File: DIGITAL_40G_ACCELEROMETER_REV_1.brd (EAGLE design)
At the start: 19 x 38 mm, 18 parts, among them IC1 ADIS16500AMLZ, IC2 LTC6820IUD#PBF, IC3 LDL1117S33R, T1 782482_33VC

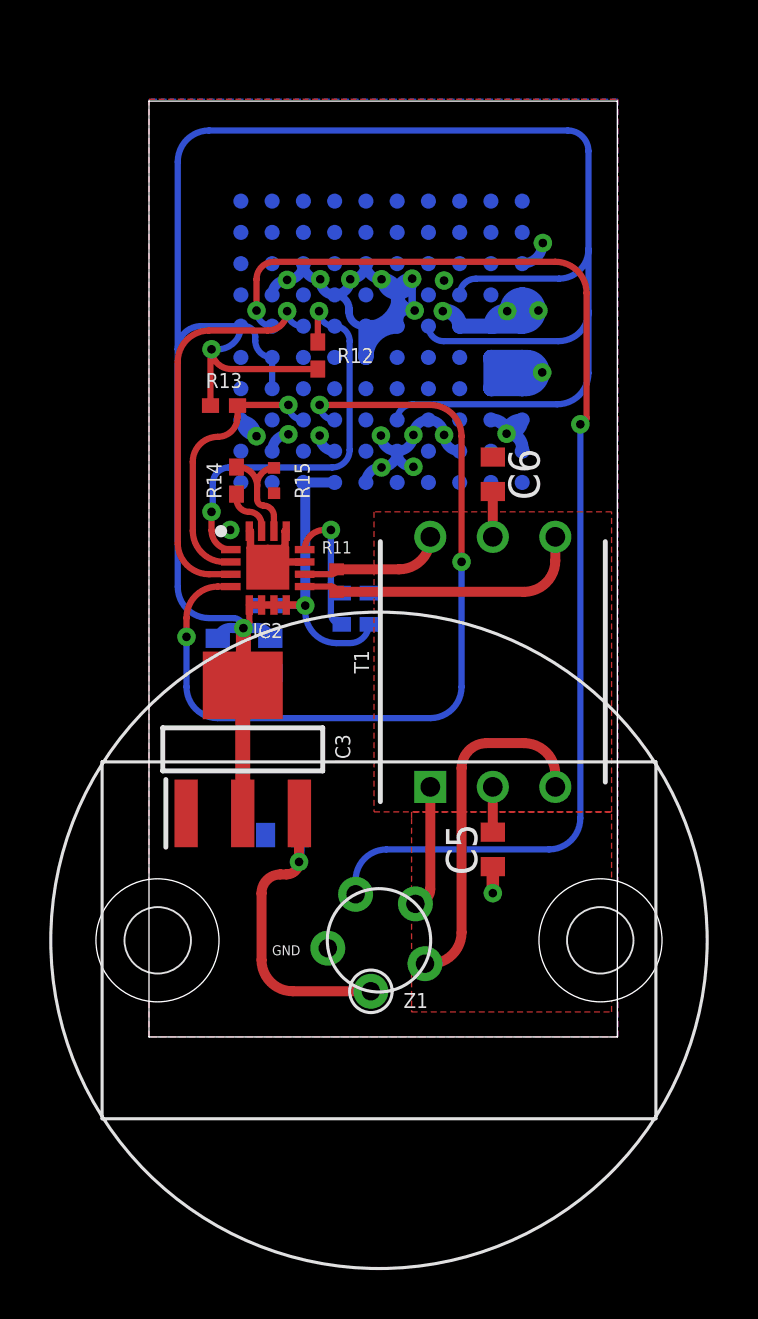
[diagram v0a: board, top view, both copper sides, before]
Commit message: Second Draft of Digital 40G Layout. Ready for review.
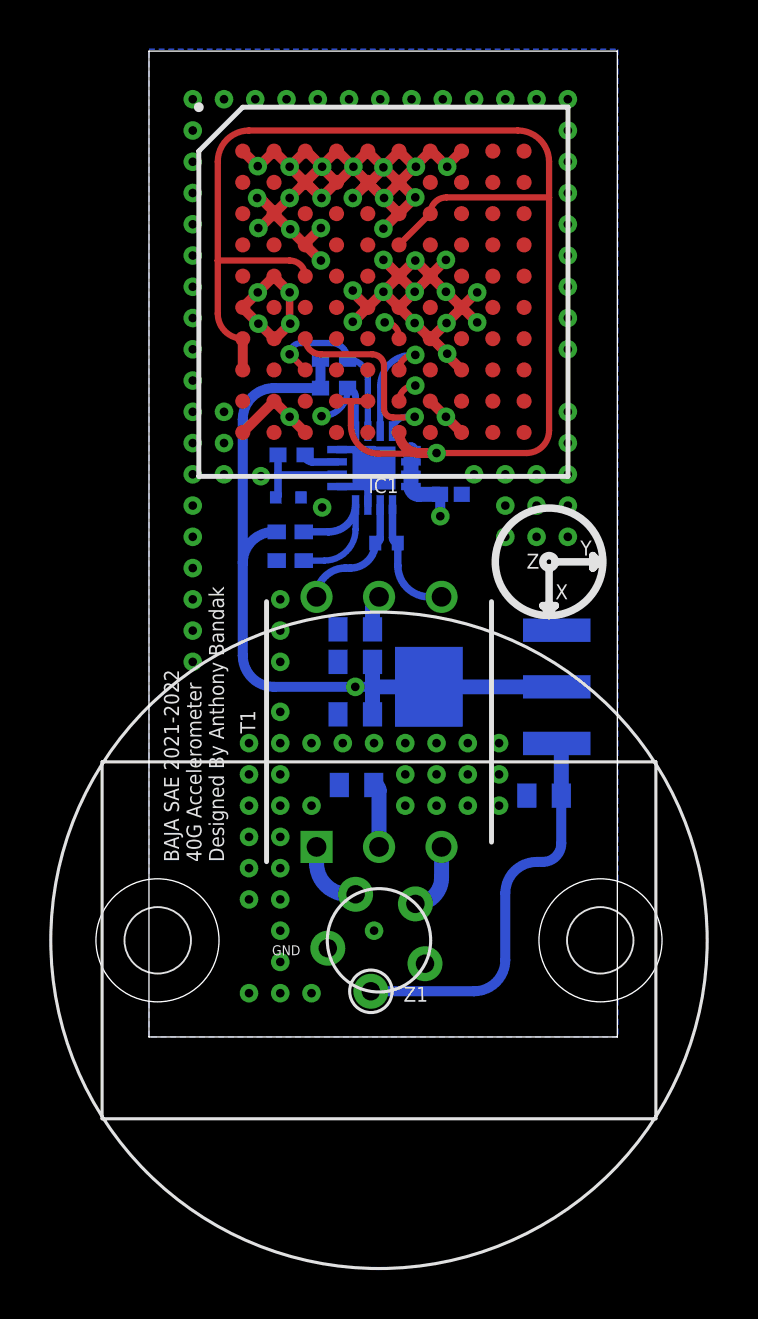
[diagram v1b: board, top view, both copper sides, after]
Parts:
- moved C1 10.7 mm to (16.1, 9.80)
- moved IC3 10.5 mm to (14.0, 14.2), flipped to the bottom, turned to 0 degrees
- moved C4 8.71 mm to (12.3, 22.0), turned to 180 degrees
- moved C6 8.42 mm to (8.38, 16.6), flipped to the bottom, turned to 0 degrees
- moved C5 6.12 mm to (8.43, 10.2), flipped to the bottom, turned to 0 degrees
- moved IC2 5.93 mm to (9.14, 23.1), flipped to the bottom, turned to 270 degrees
- moved C2 5.59 mm to (8.38, 15.2), turned to 0 degrees
- moved T1 5.23 mm to (9.35, 12.8)
- moved R13 4.85 mm to (7.52, 27.5), flipped to the bottom, turned to 0 degrees
- moved R17 4.59 mm to (5.74, 20.5), turned to 0 degrees
- moved C3 4.20 mm to (8.38, 13.1), turned to 0 degrees
- moved R16 2.95 mm to (5.74, 19.4), turned to 0 degrees
- moved R11 2.54 mm to (9.65, 20.1), flipped to the bottom, turned to 0 degrees
- moved R14 2.47 mm to (5.79, 23.6), flipped to the bottom, turned to 0 degrees
- moved IC1 2.03 mm to (9.53, 30.3), flipped to the top, turned to 0 degrees
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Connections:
- net DR: now also Z1.3; no longer Z1.5
- net IM: now also Z1.4; no longer Z1.3
- net IP: now also Z1.5; no longer Z1.4
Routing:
- net CS: track 34.7 -> 7.94 mm, vias 3 -> 1
- net DR: track 48.6 -> 35.0 mm, vias 2 -> 1
- net SCK: track 16.3 -> 4.69 mm
- net IM: track 14.0 -> 2.76 mm
- net IMBOARD: track 11.8 -> 4.86 mm
- net MOSI: track 16.6 -> 10.0 mm
- net GND: track 78.3 -> 73.4 mm, vias 23 -> 131
- net MISO: track 10.9 -> 6.98 mm
- net 12V: track 12.8 -> 16.0 mm, vias 1 -> 0
- net IP: track 5.00 -> 2.77 mm
- net IPBOARD: track 5.76 -> 4.92 mm
- net N$2: track 1.84 -> 2.60 mm
- net IBIAS: track 1.93 -> 1.42 mm
- net SLOW: track 6.04 -> 6.17 mm, vias 1 -> 0
- added copper zone on layer 15, net GND
- removed copper zone on layer 1, net GND
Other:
- board size 19 x 38 mm -> 19 x 40.1 mm
- board text added: "BAJA SAE 2021-2022 40G Accelerometer Designed By Anthony Bandak"
- board text added: "X"
- board text added: "Y"
- board text added: "Z"
